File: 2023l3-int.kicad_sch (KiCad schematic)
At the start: 14 parts, among them J1 0526101433, J2 Conn_01x03_Pin, SW1 SW_DIP_x02, U28 xiao-esp32c3

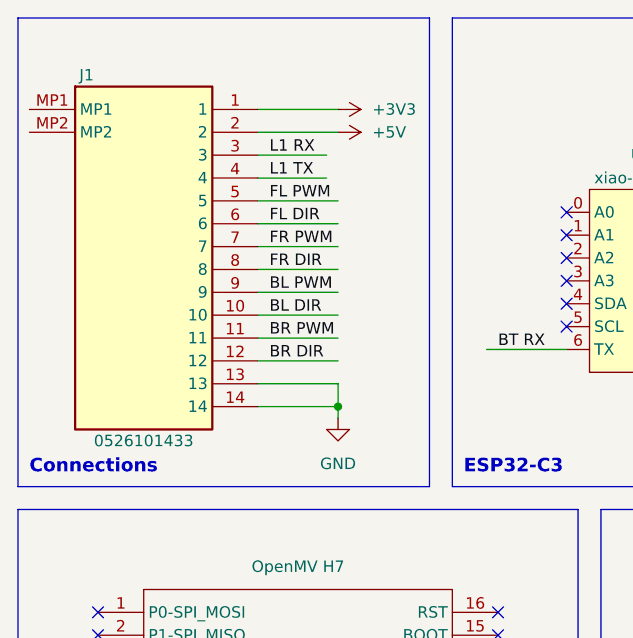
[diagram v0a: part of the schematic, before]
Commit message: final
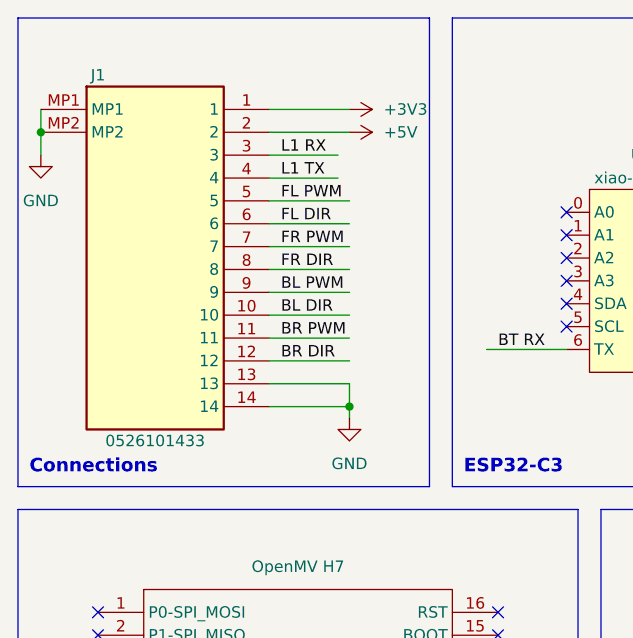
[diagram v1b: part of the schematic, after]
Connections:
- net GND: now also J1.MP1, J1.MP2
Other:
- moved on the sheet: J1
